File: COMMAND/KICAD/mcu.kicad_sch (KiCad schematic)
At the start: 10 parts

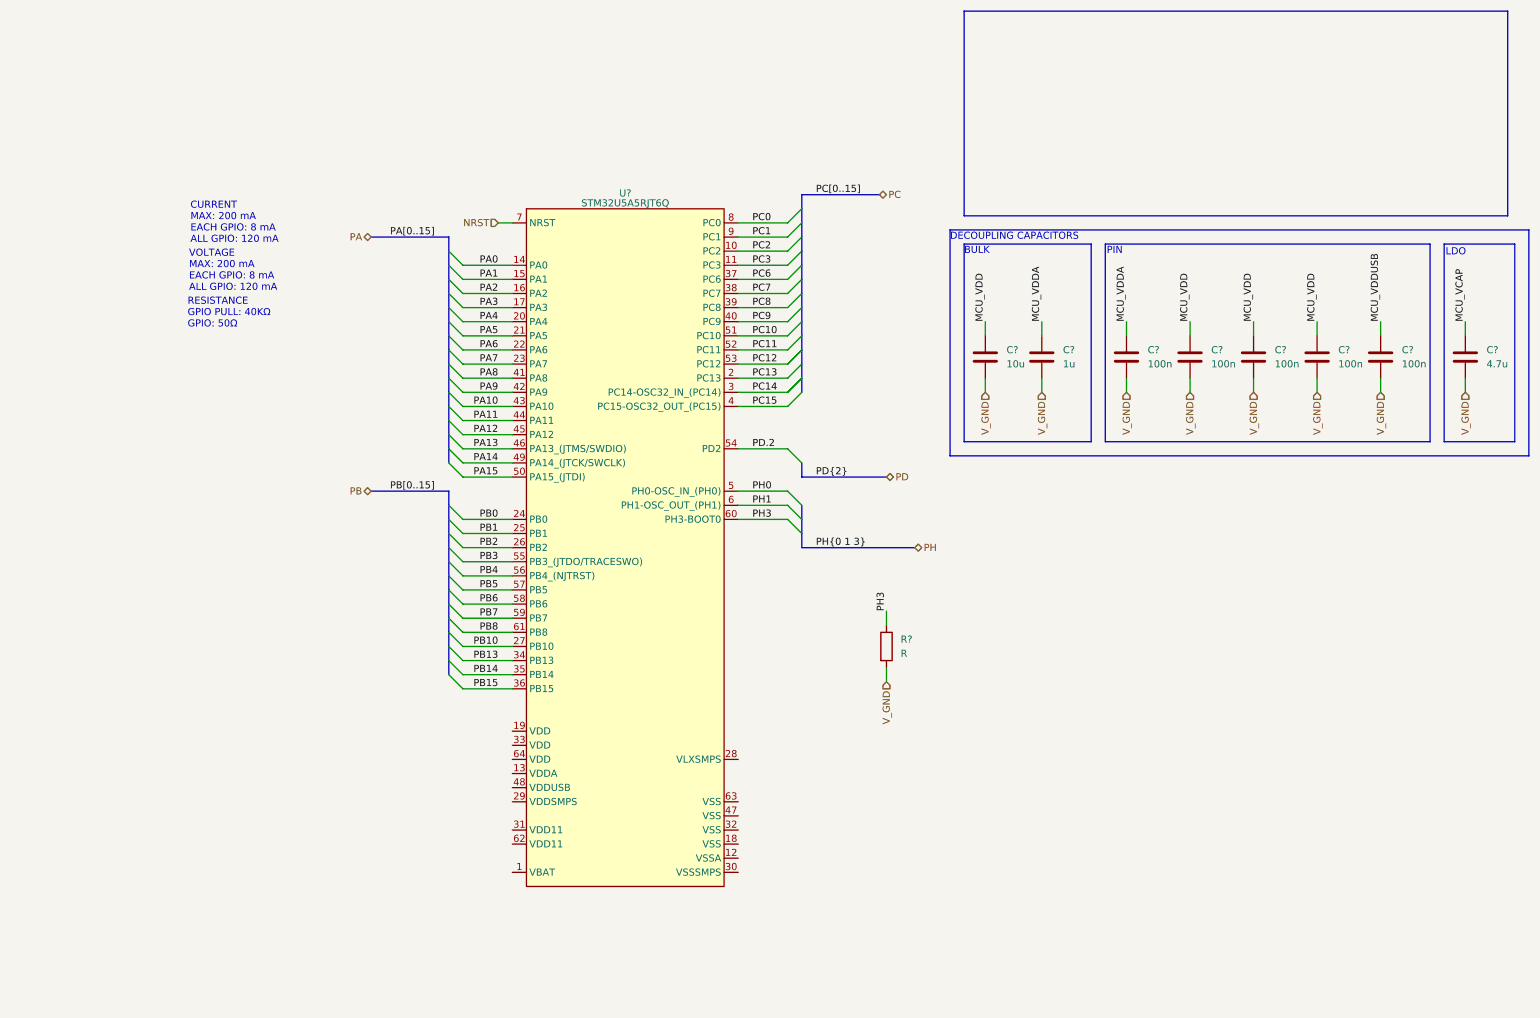
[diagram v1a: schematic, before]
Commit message: Updated Command Kicad
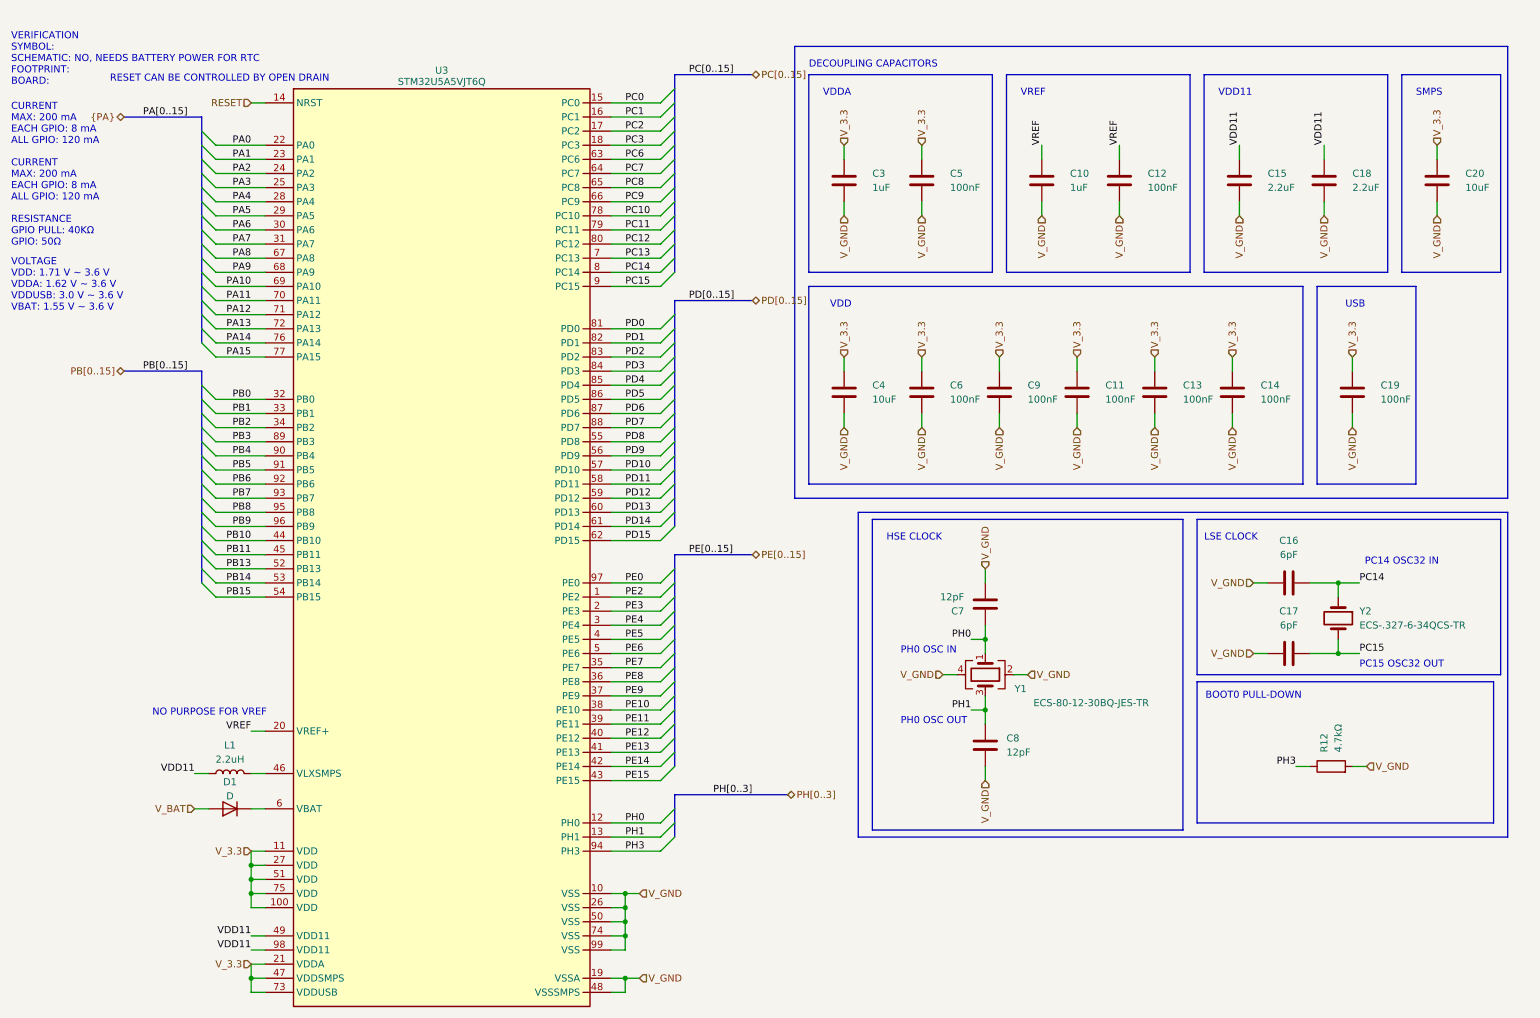
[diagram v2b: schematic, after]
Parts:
- removed C?: 1u, symbol Device:C
- removed C?: 10u, symbol Device:C
- removed C? (x5): 100n, symbol Device:C
- removed C?: 4.7u, symbol Device:C
- removed R?: R, symbol Device:R
- removed U?: STM32U5A5RJT6Q, symbol CUBESAT:STM32U5A5RJT6Q
- added C10, C3: 1uF, Capacitor_SMD:C_1206_3216Metric, symbol Device:C
- added C11, C12, C13, C14, C19, C5, C6, C9: 100nF, Capacitor_SMD:C_0603_1608Metric, symbol Device:C
- added C15, C18: 2.2uF, Capacitor_SMD:C_1206_3216Metric, symbol Device:C
- added C16, C17: 6pF, symbol Device:C
- added C20, C4: 10uF, Capacitor_SMD:C_1206_3216Metric, symbol Device:C
- added C7, C8: 12pF, symbol Device:C
- added D1: D, symbol Device:D
- added L1: 2.2uH, Inductor_SMD:L_0805_2012Metric, symbol Device:L
- added R12: 4.7kΩ, Resistor_SMD:R_0603_1608Metric, symbol Device:R
- added U3: STM32U5A5VJT6Q, CUBESAT:STM32U5A5VJ, symbol CUBESAT:STM32U5A5VJT6Q
- added Y1: ECS-80-12-30BQ-JES-TR, Crystal:Crystal_SMD_5032-4Pin_5.0x3.2mm, symbol Device:Crystal_GND24
- added Y2: ECS-.327-6-34QCS-TR, Crystal:Crystal_SMD_3215-2Pin_3.2x1.5mm, symbol Device:Crystal
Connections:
- net PA0: now also U3.22 (PA0)
- net PA1: now also U3.23 (PA1)
- net PA10: now also U3.69 (PA10)
- net PA11: now also U3.70 (PA11)
- net PA12: now also U3.71 (PA12)
- net PA13: now also U3.72 (PA13)
- net PA14: now also U3.76 (PA14)
- net PA15: now also U3.77 (PA15)
- net PA2: now also U3.24 (PA2)
- net PA3: now also U3.25 (PA3)
- net PA4: now also U3.28 (PA4)
- net PA5: now also U3.29 (PA5)
- net PA6: now also U3.30 (PA6)
- net PA7: now also U3.31 (PA7)
- net PA8: now also U3.67 (PA8)
- net PA9: now also U3.68 (PA9)
- net PB0: now also U3.32 (PB0)
- net PB1: now also U3.33 (PB1)
- net PB10: now also U3.44 (PB10)
- net PB13: now also U3.52 (PB13)
- net PB14: now also U3.53 (PB14)
- net PB15: now also U3.54 (PB15)
- net PB2: now also U3.34 (PB2)
- net PB3: now also U3.89 (PB3)
- net PB4: now also U3.90 (PB4)
- net PB5: now also U3.91 (PB5)
- net PB6: now also U3.92 (PB6)
- net PB7: now also U3.93 (PB7)
- net PB8: now also U3.95 (PB8)
- net PC0: now also U3.15 (PC0)
- net PC1: now also U3.16 (PC1)
- net PC10: now also U3.78 (PC10)
- net PC11: now also U3.79 (PC11)
- net PC12: now also U3.80 (PC12)
- net PC13: now also U3.7 (PC13)
- net PC14: now also C16.1, U3.8 (PC14), Y2.1
- net PC15: now also C17.1, U3.9 (PC15), Y2.2
- net PC2: now also U3.17 (PC2)
- net PC3: now also U3.18 (PC3)
- net PC6: now also U3.63 (PC6)
- net PC7: now also U3.64 (PC7)
- net PC8: now also U3.65 (PC8)
- net PC9: now also U3.66 (PC9)
- net PH0: now also C7.1, U3.12 (PH0), Y1.1
- net PH1: now also C8.1, U3.13 (PH1), Y1.3
- net PH3: now also R12.1, U3.94 (PH3)
- net V_GND: now also C10.2, C11.2, C12.2, C13.2, C14.2, C15.2, C16.2, C17.2, C18.2, C19.2, C20.2, C3.2, C4.2, C5.2, C6.2, C7.2, C8.2, C9.2, R12.2, U3.10 (VSS), U3.19 (VSSA), U3.26 (VSS), U3.48 (VSSSMPS), U3.50 (VSS), U3.74 (VSS), U3.99 (VSS), Y1.2, Y1.4
- new net: D1.1 (K), U3.6 (VBAT)
- new net: L1.2, U3.46 (VLXSMPS)
- new net PB11: U3.45 (PB11)
- new net PB9: U3.96 (PB9)
- new net PD0: U3.81 (PD0)
- new net PD1: U3.82 (PD1)
- new net PD10: U3.57 (PD10)
- new net PD11: U3.58 (PD11)
- new net PD12: U3.59 (PD12)
- new net PD13: U3.60 (PD13)
- new net PD14: U3.61 (PD14)
- new net PD15: U3.62 (PD15)
- new net PD2: U3.83 (PD2)
- new net PD3: U3.84 (PD3)
- new net PD4: U3.85 (PD4)
- new net PD5: U3.86 (PD5)
- new net PD6: U3.87 (PD6)
- new net PD7: U3.88 (PD7)
- new net PD8: U3.55 (PD8)
- new net PD9: U3.56 (PD9)
- new net PE0: U3.97 (PE0)
- new net PE10: U3.38 (PE10)
- new net PE11: U3.39 (PE11)
- new net PE12: U3.40 (PE12)
- new net PE13: U3.41 (PE13)
- new net PE14: U3.42 (PE14)
- new net PE15: U3.43 (PE15)
- new net PE2: U3.1 (PE2)
- new net PE3: U3.2 (PE3)
- new net PE4: U3.3 (PE4)
- new net PE5: U3.4 (PE5)
- new net PE6: U3.5 (PE6)
- new net PE7: U3.35 (PE7)
- new net PE8: U3.36 (PE8)
- new net PE9: U3.37 (PE9)
- new net RESET: U3.14 (NRST)
- new net VDD11: C15.1, C18.1, L1.1, U3.49 (VDD11), U3.98 (VDD11)
- new net VREF: C10.1, C12.1, U3.20 (VREF+)
- new net V_3.3: C11.1, C13.1, C14.1, C19.1, C20.1, C3.1, C4.1, C5.1, C6.1, C9.1, U3.100 (VDD), U3.11 (VDD), U3.21 (VDDA), U3.27 (VDD), U3.47 (VDDSMPS), U3.51 (VDD), U3.73 (VDDUSB), U3.75 (VDD)
- new net V_BAT: D1.2 (A)
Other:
- note added: "BOOT0 PULL-DOWN"
- note added: "HSE CLOCK"
- note added: "LSE CLOCK"
- note added: "NO PURPOSE FOR VREF"
- note added: "PC14 OSC32 IN"
- note added: "PC15 OSC32 OUT"
- note added: "PH0 OSC IN"
- note added: "PH0 OSC OUT"
- note added: "RESET CAN BE CONTROLLED BY OPEN DRAIN"
- note added: "SMPS"
- note added: "USB"
- note added: "VDD"
- note added: "VDD11"
- note added: "VDDA"
- note added: "VERIFICATION SYMBOL: SCHEMATIC: NO, NEEDS BATTERY POWER FOR RTC FOOTPRINT: BOARD:"
- note added: "VOLTAGE VDD: 1.71 V ~ 3.6 V VDDA: 1.62 V ~ 3.6 V VDDUSB: 3.0 V ~ 3.6 V VBAT: 1.55 V ~ 3.6 V"
- note added: "VREF"
- note removed: "BULK"
- note removed: "LDO"
- note removed: "PIN"
- note removed: "VOLTAGE MAX: 200 mA EACH GPIO: 8 mA ALL GPIO: 120 mA"
